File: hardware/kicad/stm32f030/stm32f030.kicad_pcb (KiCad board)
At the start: 2 copper layers, 110 parts, among them K1 RELAY_1RT, K2 RELAY_1RT, P1 5VIN, P10 SWD, P2 LOOP1, P3 LOOP2, P4 RELAY OUT 1, P5 TTL OUT 1, P6 RELAY OUT 2, P7 TTL OUT 2, P8 UART, P9 I2C, Q1 BSS138, Q2 BC817-40, Q3 BSS138, Q4 BC817-40, Q5 BC817-40, Q6 BC817-40, Q7 BC817-40, Q8 BC817-40, SW1 TACTILE_SW, SW2 TACTILE_SW, SW3 RESET, T1 78601/9C, T2 78601/9C, U1 LM1117-3.3, U2 STM32F030F4Px, U3 MCP23017, Y1 8MHz

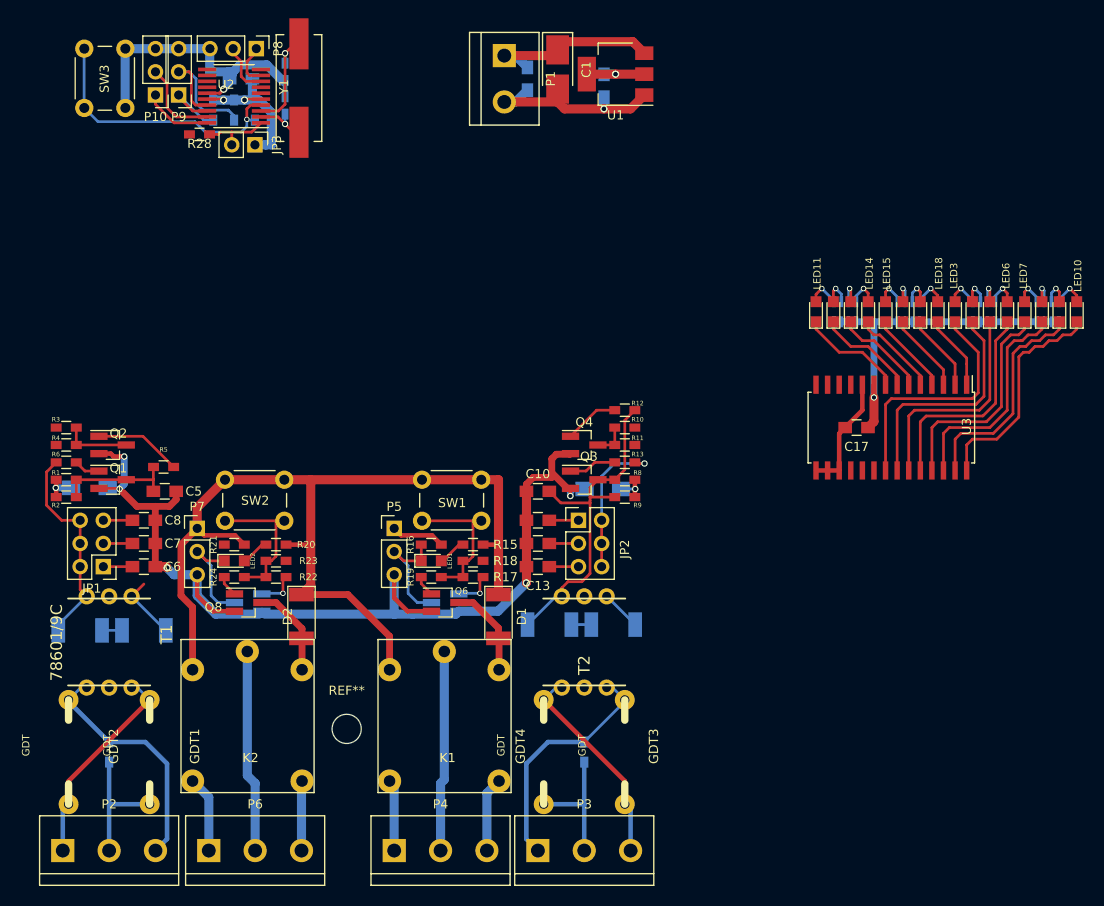
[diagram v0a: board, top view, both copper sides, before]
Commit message: PCB V0.90
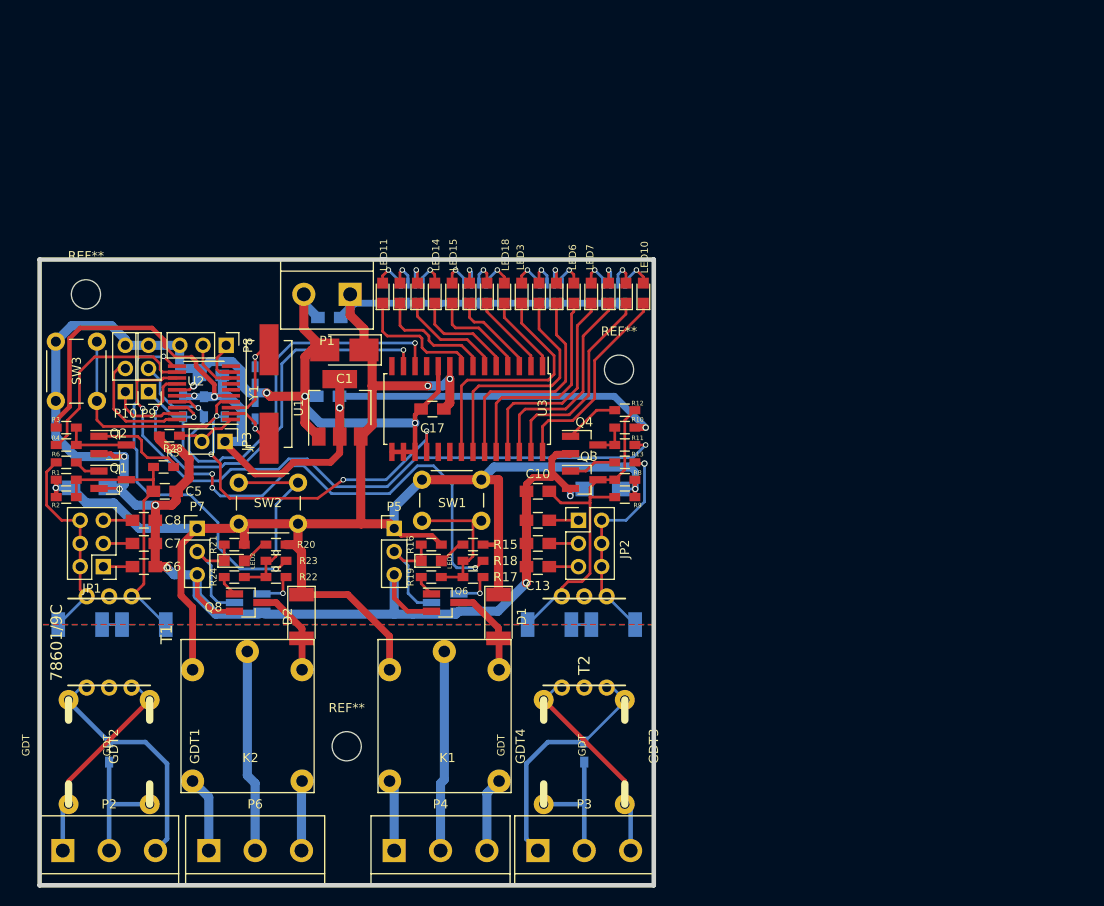
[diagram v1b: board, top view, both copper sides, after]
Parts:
- added REF**: MountingHole_3.2mm_M3, Mounting_Holes:MountingHole_3.2mm_M3, F.Cu at (40.6, 96.5)
- added REF**: MountingHole_3.2mm_M3, Mounting_Holes:MountingHole_3.2mm_M3, F.Cu at (99.1, 104.8)
- moved LED17 47.5 mm to (84.6, 96.4)
- moved LED18 47.5 mm to (86.5, 96.4)
- moved LED11 47.5 mm to (73.2, 96.4)
- moved LED12 47.5 mm to (75.1, 96.4)
- moved LED15 47.5 mm to (80.8, 96.4)
- moved LED16 47.5 mm to (82.7, 96.4)
- moved RN1 47.5 mm to (91.6, 96.4)
- moved RN2 47.5 mm to (98.6, 96.4)
- moved RN3 47.5 mm to (76.3, 96.4)
- moved RN4 47.5 mm to (83.3, 96.4)
- moved LED10 47.5 mm to (101.7, 96.4)
- moved LED13 47.5 mm to (77.0, 96.4)
- moved LED14 47.5 mm to (78.9, 96.4)
- moved LED3 47.5 mm to (88.4, 96.4)
- moved LED4 47.5 mm to (90.3, 96.4)
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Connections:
- P10 pad 1: /MCU/SWC -> /MCU/SWD
- P10 pad 2: /MCU/SWD -> /MCU/SWC
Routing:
- net +3V3: track 26.1 -> 110.6 mm, vias 3 -> 4
- net /colpitts/osc1: track 0.00 -> 73.3 mm, vias 0 -> 2
- net /outputs/active1: track 0.00 -> 61.0 mm, vias 0 -> 4
- net GND: track 184.6 -> 234.0 mm, vias 7 -> 10
- net +5V: track 175.0 -> 218.2 mm, vias 3 -> 4
- net /MCU/active1: track 0.00 -> 40.9 mm, vias 0 -> 2
- net /MCU/sda: track 9.19 -> 49.3 mm, vias 0 -> 2
- net /MCU/scl: track 16.5 -> 53.9 mm, vias 0 -> 2
- net /MCU/reset: track 30.2 -> 63.7 mm, vias 1 -> 4
- net /MCU/osc1: track 0.00 -> 21.6 mm
- net Net-(C5-Pad1): track 20.3 -> 30.6 mm
- net /MCU/SWC: track 7.52 -> 13.0 mm
- net Net-(R22-Pad2): track 15.8 -> 21.0 mm, vias 0 -> 1
- net Net-(JP2-Pad2): track 20.7 -> 23.8 mm
- net Net-(LED11-Pad1): track 11.5 -> 14.5 mm
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- added copper zone on B.Cu, net GND
- added copper zone on F.Cu, net GND
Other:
- board outline added: 67.3 x 68.6 mm
